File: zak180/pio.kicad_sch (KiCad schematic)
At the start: 25 parts, among them J2 DB25_Receptacle_MountingHoles, U2 PIO-DIP-40

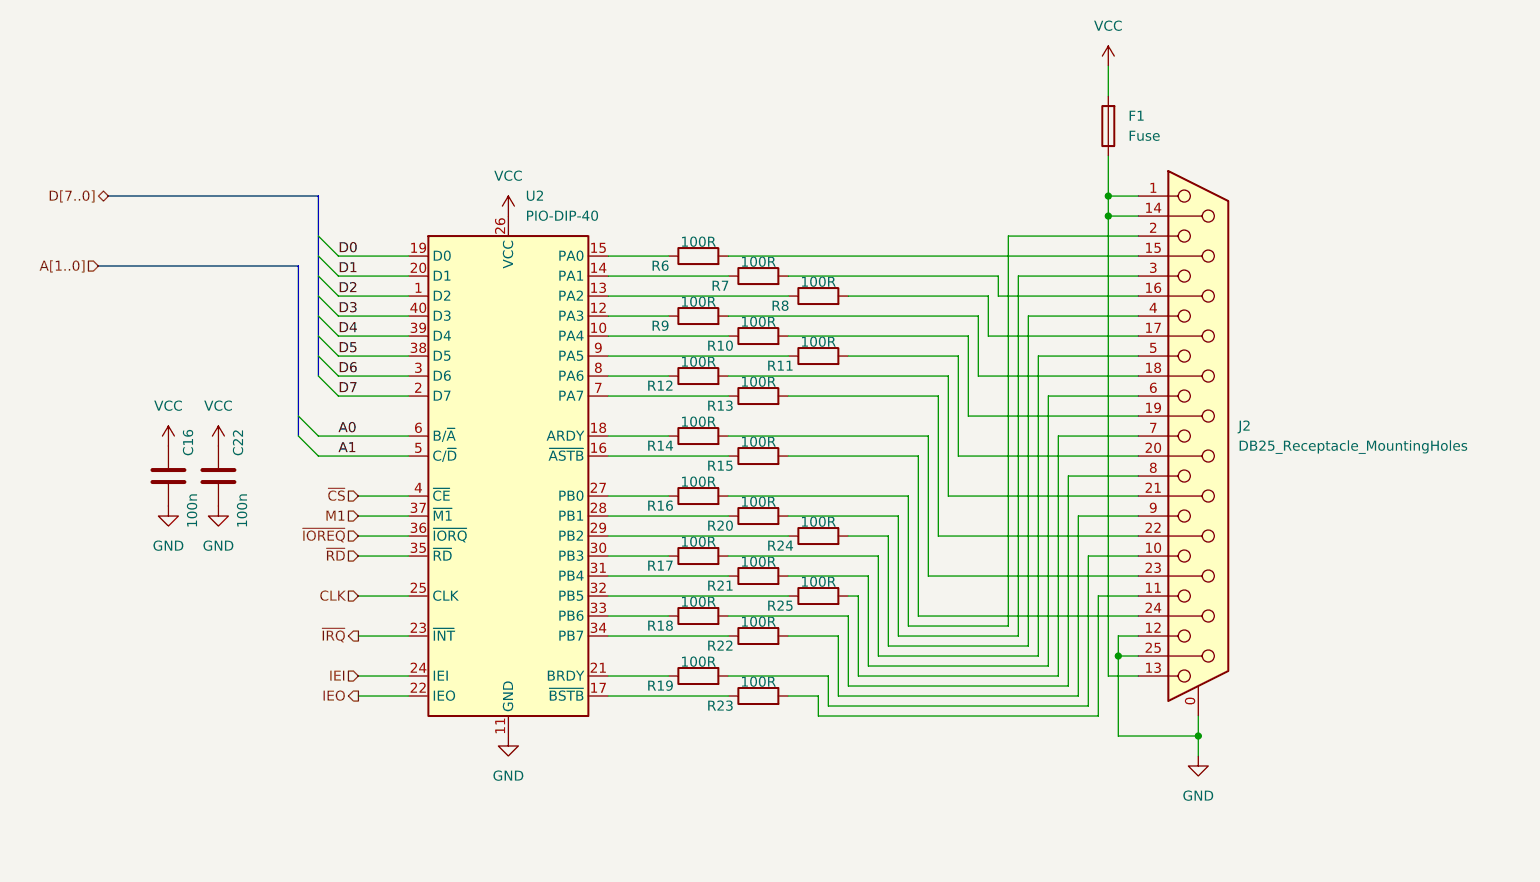
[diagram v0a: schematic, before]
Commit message: HW: PCB complete
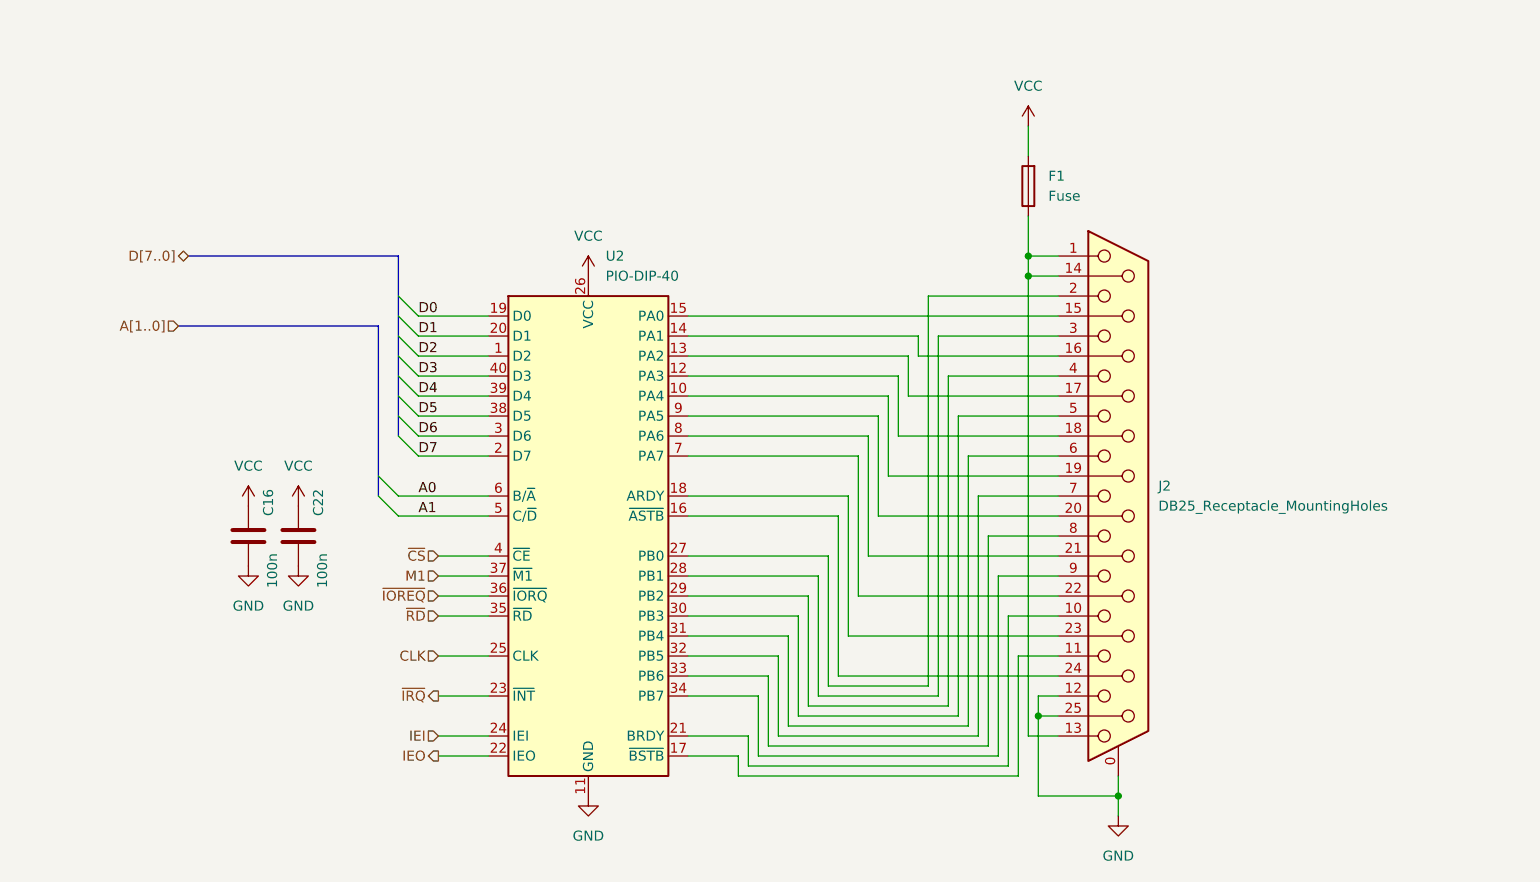
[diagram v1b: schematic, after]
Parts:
- removed R10, R11, R12, R13, R14, R15, R16, R17, R18, R19, R20, R21, R22, R23, R24, R25, R6, R7, R8, R9: 100R, Resistor_THT:R_Axial_DIN0207_L6.3mm_D2.5mm_P7.62mm_Horizontal, symbol Device:R
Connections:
- net at U2.28 (PB1): now also J2.3
- net at U2.9 (PA5): now also J2.20 (P20)
- net at U2.13 (PA2): now also J2.17 (P17)
- net at U2.33 (PB6): now also J2.8
- net at U2.17 (~{BSTB}): now also J2.11
- net at J2.10: now also U2.21 (BRDY)
- net at J2.15 (P15): now also U2.15 (PA0)
- net at J2.16 (P16): now also U2.14 (PA1)
- net at J2.18 (P18): now also U2.12 (PA3)
- net at J2.19 (P19): now also U2.10 (PA4)
- net at J2.2: now also U2.27 (PB0)
- net at J2.21 (P21): now also U2.8 (PA6)
- net at J2.22 (P22): now also U2.7 (PA7)
- net at J2.23 (P23): now also U2.18 (ARDY)
- net at J2.24 (P24): now also U2.16 (~{ASTB})
- net at J2.4: now also U2.29 (PB2)
- net at J2.5: now also U2.30 (PB3)
- net at J2.6: now also U2.31 (PB4)
- net at J2.7: now also U2.32 (PB5)
- net at J2.9: now also U2.34 (PB7)
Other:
- moved on the sheet: C16, C22, F1, J2, U2
